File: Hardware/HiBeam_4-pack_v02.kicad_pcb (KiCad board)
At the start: 2 copper layers, 21.6 x 21.6 mm, 22 parts, among them J1 5V, J2 CI, J3 DI, J4 GND, J5 CO, J6 DO, J7 5V, J8 GND, U1 APA102C, U2 APA102C, U3 APA102C, U4 APA102C

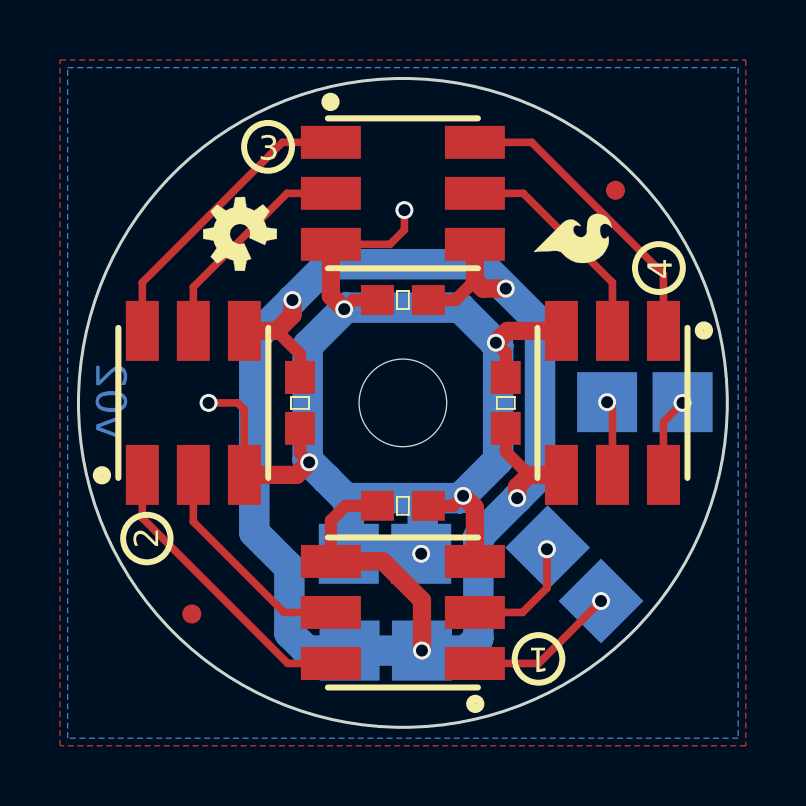
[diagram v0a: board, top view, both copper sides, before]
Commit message: Silk fixes.
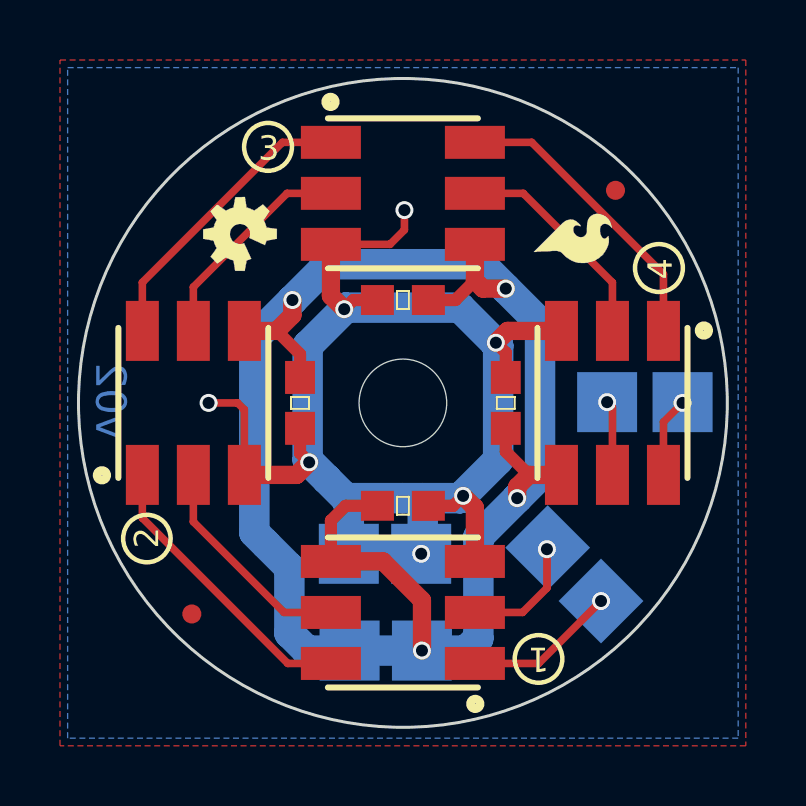
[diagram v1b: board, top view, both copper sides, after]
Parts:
- ?: footprint SparkFun:SFE_LOGO_NAME_.1 -> Aesthetics:SFE_LOGO_NAME_FLAME_.1
- moved ? 1.15 mm to (151.6, 93.3)
